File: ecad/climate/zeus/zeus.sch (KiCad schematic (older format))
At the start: 12 parts, among them J1 MCV 1,5/ 2-G-3,5, J10 47053-1000, J11 47053-1000, J12 PT 1,5/4-3,5-H, J13 PT 1,5/4-3,5-H, J2 MCV 1,5/ 2-G-3,5, J3 MCV 1,5/ 2-G-3,5, J5 47053-1000, J6 47053-1000, J7 215079-8, J8 640454-2, J9 640454-2

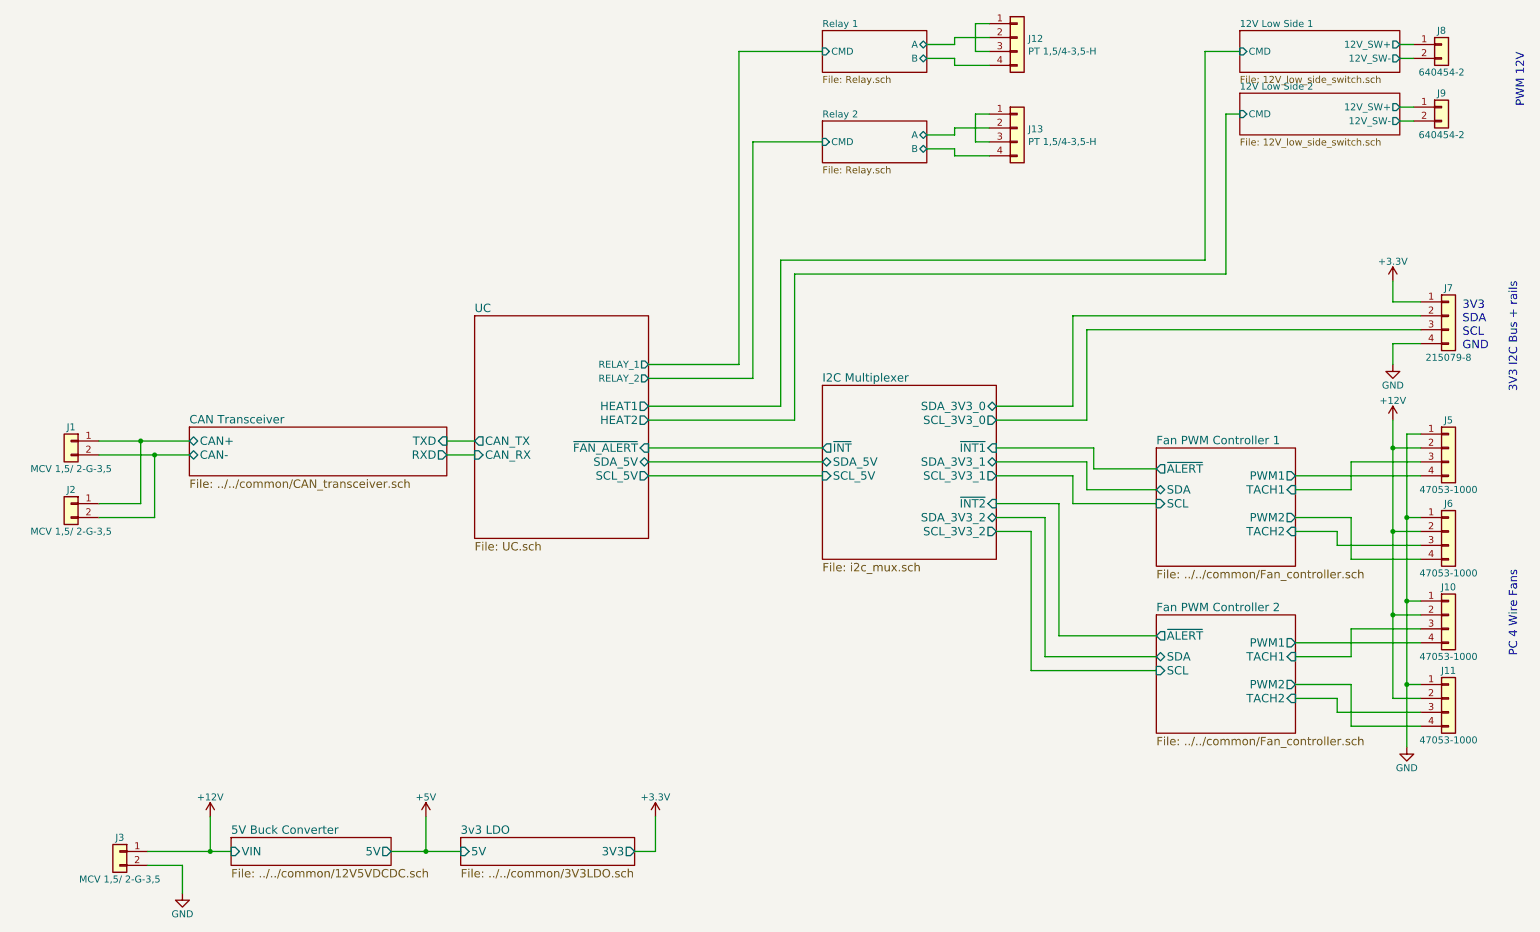
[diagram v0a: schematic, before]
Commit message: Makes pleiades zeus again
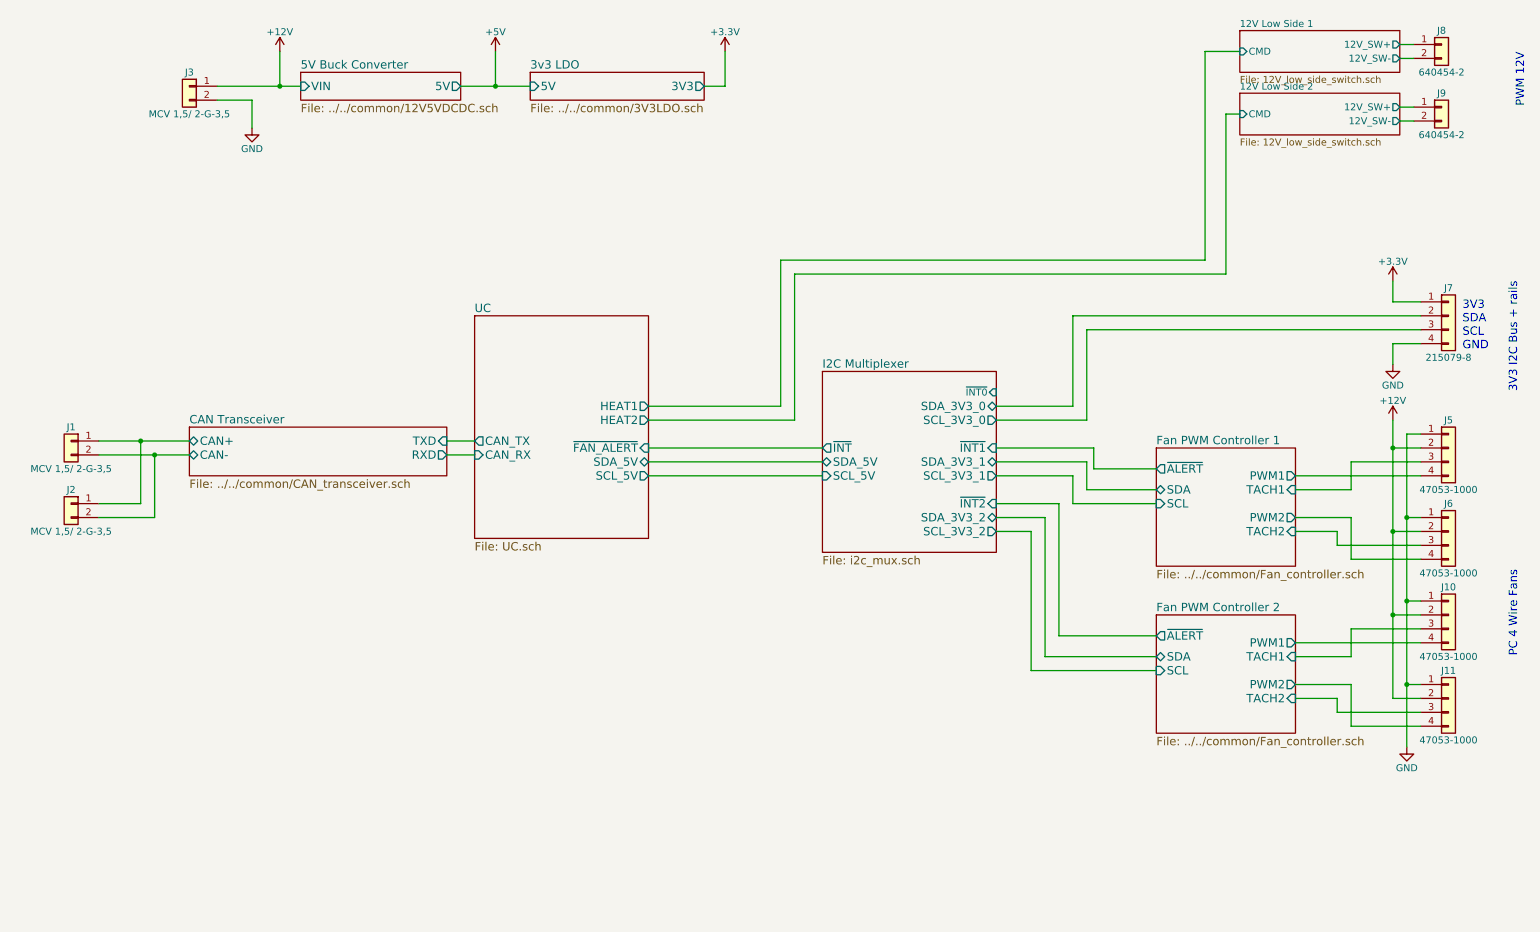
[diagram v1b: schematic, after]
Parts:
- removed J12, J13: PT 1,5/4-3,5-H, TerminalBlock_Phoenix:TerminalBlock_Phoenix_PT-1,5-4-3.5-H_1x04_P3.50mm_Horizontal, symbol Connector_Generic:Conn_01x04
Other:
- moved on the sheet: J3
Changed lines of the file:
@@
 EESchema Schematic File Version 4
-LIBS:pleiades-cache
+LIBS:zeus-cache
 EELAYER 26 0
 EELAYER END
 $Descr A4 11693 8268
 encoding utf-8
-Sheet 1 12
+Sheet 1 10
 Title ""
 Date ""
@@
 L power:+12V #PWR01
 U 1 1 5BA4C0F9
-P 1700 6750
-F 0 "#PWR01" H 1700 6600 50  0001 C CNN
-F 1 "+12V" H 1700 6890 50  0000 C CNN
-F 2 "" H 1700 6750 50  0001 C CNN
-F 3 "" H 1700 6750 50  0001 C CNN
-	1    1700 6750
+P 2200 1250
+F 0 "#PWR01" H 2200 1100 50  0001 C CNN
+F 1 "+12V" H 2200 1390 50  0000 C CNN
+F 2 "" H 2200 1250 50  0001 C CNN
+F 3 "" H 2200 1250 50  0001 C CNN
+	1    2200 1250
 	1    0    0    -1
 $EndComp
@@
 L power:+5V #PWR02
 U 1 1 5BA4C12E
-P 3250 6750
-F 0 "#PWR02" H 3250 6600 50  0001 C CNN
-F 1 "+5V" H 3250 6890 50  0000 C CNN
-F 2 "" H 3250 6750 50  0001 C CNN
-F 3 "" H 3250 6750 50  0001 C CNN
-	1    3250 6750
+P 3750 1250
+F 0 "#PWR02" H 3750 1100 50  0001 C CNN
+F 1 "+5V" H 3750 1390 50  0000 C CNN
+F 2 "" H 3750 1250 50  0001 C CNN
+F 3 "" H 3750 1250 50  0001 C CNN
+	1    3750 1250
 	1    0    0    -1
 $EndComp
@@
 $EndSheet
 $Sheet
-S 3500 6900 1250 200
+S 4000 1400 1250 200
 U 5BA4EFD7
 F0 "3v3 LDO" 60
 F1 "../../common/3V3LDO.sch" 60
-F2 "5V" I L 3500 7000 60
-F3 "3V3" O R 4750 7000 60
-$EndSheet
-$Sheet
-S 1850 6900 1150 200
+F2 "5V" I L 4000 1500 60
+F3 "3V3" O R 5250 1500 60
+$EndSheet
+$Sheet
+S 2350 1400 1150 200
 U 5BA4BC5D
 F0 "5V Buck Converter" 60
 F1 "../../common/12V5VDCDC.sch" 60
-F2 "VIN" I L 1850 7000 60
-F3 "5V" O R 3000 7000 60
+F2 "VIN" I L 2350 1500 60
+F3 "5V" O R 3500 1500 60
 $EndSheet
 $Comp
 L pleiades-rescue:+3.3V #PWR03
 U 1 1 5BA4FC58
-P 4900 6750
-F 0 "#PWR03" H 4900 6600 50  0001 C CNN
-F 1 "+3.3V" H 4900 6890 50  0000 C CNN
-F 2 "" H 4900 6750 50  0001 C CNN
-F 3 "" H 4900 6750 50  0001 C CNN
-	1    4900 6750
+P 5400 1250
+F 0 "#PWR03" H 5400 1100 50  0001 C CNN
+F 1 "+3.3V" H 5400 1390 50  0000 C CNN
+F 2 "" H 5400 1250 50  0001 C CNN
+F 3 "" H 5400 1250 50  0001 C CNN
+	1    5400 1250
 	1    0    0    -1
 $EndComp
@@
 L Connector_Generic:Conn_01x02 J3
 U 1 1 5BA567FD
-P 1050 7000
-F 0 "J3" H 1050 7100 50  0000 C CNN
-F 1 "MCV 1,5/ 2-G-3,5" H 1050 6800 50  0000 C CNN
-F 2 "Connector_Phoenix_MC:PhoenixContact_MCV_1,5_2-G-3.5_1x02_P3.50mm_Vertical" H 1050 7000 50  0001 C CNN
-F 3 "" H 1050 7000 50  0001 C CNN
-F 4 "MCV 1,5/ 2-G-3,5" H 1050 7000 60  0001 C CNN "Part Number"
-	1    1050 7000
+P 1550 1500
+F 0 "J3" H 1550 1600 50  0000 C CNN
+F 1 "MCV 1,5/ 2-G-3,5" H 1550 1300 50  0000 C CNN
+F 2 "Connector_Phoenix_MC:PhoenixContact_MCV_1,5_2-G-3.5_1x02_P3.50mm_Vertical" H 1550 1500 50  0001 C CNN
+F 3 "" H 1550 1500 50  0001 C CNN
+F 4 "MCV 1,5/ 2-G-3,5" H 1550 1500 60  0001 C CNN "Part Number"
+	1    1550 1500
 	-1   0    0    -1
 $EndComp
@@
 L power:GND #PWR08
 U 1 1 5BA570D8
-P 1500 7300
-F 0 "#PWR08" H 1500 7050 50  0001 C CNN
-F 1 "GND" H 1500 7150 50  0000 C CNN
-F 2 "" H 1500 7300 50  0001 C CNN
-F 3 "" H 1500 7300 50  0001 C CNN
-	1    1500 7300
+P 2000 1800
+F 0 "#PWR08" H 2000 1550 50  0001 C CNN
+F 1 "GND" H 2000 1650 50  0000 C CNN
+F 2 "" H 2000 1800 50  0001 C CNN
+F 3 "" H 2000 1800 50  0001 C CNN
+	1    2000 1800
 	1    0    0    -1
 $EndComp
@@
 F7 "SDA_5V" B R 4850 4200 60
 F8 "SCL_5V" O R 4850 4300 60
-F9 "RELAY_1" O R 4850 3500 50
-F10 "RELAY_2" O R 4850 3600 50
 $EndSheet
 $Sheet
@@
 $EndComp
 Wire Wire Line
-	1700 6750 1700 7000
-Wire Wire Line
-	1250 7000 1700 7000
-Wire Wire Line
-	3000 7000 3250 7000
-Wire Wire Line
-	3250 7000 3250 6750
-Connection ~ 3250 7000
-Wire Wire Line
-	4750 7000 4900 7000
-Wire Wire Line
-	4900 7000 4900 6750
+	2200 1250 2200 1500
+Wire Wire Line
+	1750 1500 2200 1500
+Wire Wire Line
+	3500 1500 3750 1500
+Wire Wire Line
+	3750 1500 3750 1250
+Connection ~ 3750 1500
+Wire Wire Line
+	5250 1500 5400 1500
+Wire Wire Line
+	5400 1500 5400 1250
 Wire Wire Line
 	10300 4600 10400 4600
@@
 	1300 4600 900  4600
 Connection ~ 1300 4150
-Connection ~ 1700 7000
-Wire Wire Line
-	1250 7100 1500 7100
-Wire Wire Line
-	1500 7100 1500 7300
+Connection ~ 2200 1500
+Wire Wire Line
+	1750 1600 2000 1600
+Wire Wire Line
+	2000 1600 2000 1800
 Wire Wire Line
 	3400 4050 3600 4050
@@
 	7800 5450 8500 5450
 $Sheet
-S 6100 3650 1250 1250
+S 6100 3550 1250 1300
 U 5BAB6A7C
 F0 "I2C Multiplexer" 60
@@
 F11 "~INT1" I R 7350 4100 60
 F12 "~INT2" I R 7350 4500 60
+F13 "~INT0" I R 7350 3700 50
 $EndSheet
 Wire Wire Line
@@
 	7600 5700 8500 5700
 Wire Wire Line
-	3250 7000 3500 7000
+	3750 1500 4000 1500
 Wire Wire Line
 	10200 4100 10200 4700
@@
 	1300 4150 1550 4150
 Wire Wire Line
-	1700 7000 1850 7000
+	2200 1500 2350 1500
 Wire Wire Line
 	10300 5800 10300 5200
@@
 Wire Wire Line
 	10250 1300 10350 1300
-$Sheet
-S 6100 1100 750  300
-U 5BB4177A
-F0 "Relay 1" 50
-F1 "Relay.sch" 50
-F2 "CMD" I L 6100 1250 50
-F3 "A" B R 6850 1200 50
-F4 "B" B R 6850 1300 50
-$EndSheet
-$Comp
-L Connector_Generic:Conn_01x04 J12
-U 1 1 5BB464E2
-P 7500 1150
-F 0 "J12" H 7579 1142 50  0000 L CNN
-F 1 "PT 1,5/4-3,5-H" H 7579 1051 50  0000 L CNN
-F 2 "TerminalBlock_Phoenix:TerminalBlock_Phoenix_PT-1,5-4-3.5-H_1x04_P3.50mm_Horizontal" H 7500 1150 50  0001 C CNN
-F 3 "~" H 7500 1150 50  0001 C CNN
-F 4 "PT 1,5/4-3,5-H" H 7500 1150 50  0001 C CNN "Part Number"
-	1    7500 1150
-	1    0    0    -1
-$EndComp
-Wire Wire Line
-	7300 1050 7200 1050
-Wire Wire Line
-	7200 1050 7200 1250
-Wire Wire Line
-	7200 1250 7300 1250
-Wire Wire Line
-	6850 1200 7050 1200
-Wire Wire Line
-	7050 1200 7050 1150
-Wire Wire Line
-	7050 1150 7300 1150
-Wire Wire Line
-	6850 1300 7050 1300
-Wire Wire Line
-	7050 1300 7050 1350
-Wire Wire Line
-	7050 1350 7300 1350
-$Sheet
-S 6100 1750 750  300
-U 5BB53554
-F0 "Relay 2" 50
-F1 "Relay.sch" 50
-F2 "CMD" I L 6100 1900 50
-F3 "A" B R 6850 1850 50
-F4 "B" B R 6850 1950 50
-$EndSheet
-$Comp
-L Connector_Generic:Conn_01x04 J13
-U 1 1 5BB5355B
-P 7500 1800
-F 0 "J13" H 7579 1792 50  0000 L CNN
-F 1 "PT 1,5/4-3,5-H" H 7579 1701 50  0000 L CNN
-F 2 "TerminalBlock_Phoenix:TerminalBlock_Phoenix_PT-1,5-4-3.5-H_1x04_P3.50mm_Horizontal" H 7500 1800 50  0001 C CNN
-F 3 "~" H 7500 1800 50  0001 C CNN
-F 4 "PT 1,5/4-3,5-H" H 7500 1800 50  0001 C CNN "Part Number"
-	1    7500 1800
-	1    0    0    -1
-$EndComp
-Wire Wire Line
-	7300 1700 7200 1700
-Wire Wire Line
-	7200 1700 7200 1900
-Wire Wire Line
-	7200 1900 7300 1900
-Wire Wire Line
-	6850 1850 7050 1850
-Wire Wire Line
-	7050 1850 7050 1800
-Wire Wire Line
-	7050 1800 7300 1800
-Wire Wire Line
-	6850 1950 7050 1950
-Wire Wire Line
-	7050 1950 7050 2000
-Wire Wire Line
-	7050 2000 7300 2000
 Wire Wire Line
 	4850 4100 6100 4100
@@
 Wire Wire Line
 	8850 1250 9100 1250
-Wire Wire Line
-	4850 3600 5600 3600
-Wire Wire Line
-	5600 3600 5600 1900
-Wire Wire Line
-	5600 1900 6100 1900
-Wire Wire Line
-	4850 3500 5500 3500
-Wire Wire Line
-	5500 3500 5500 1250
-Wire Wire Line
-	5500 1250 6100 1250
 $EndSCHEMATC
